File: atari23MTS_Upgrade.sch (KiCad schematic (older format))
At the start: 37 parts, among them P1 CONN_01X01, P2 CONN_01X01, P3 CONN_01X01, P4 CONN_01X01, P5 CONN_01X01, SW1 SW_PUSH, U1 NCP1117ST33T3G, U2 STM32F401RCTx

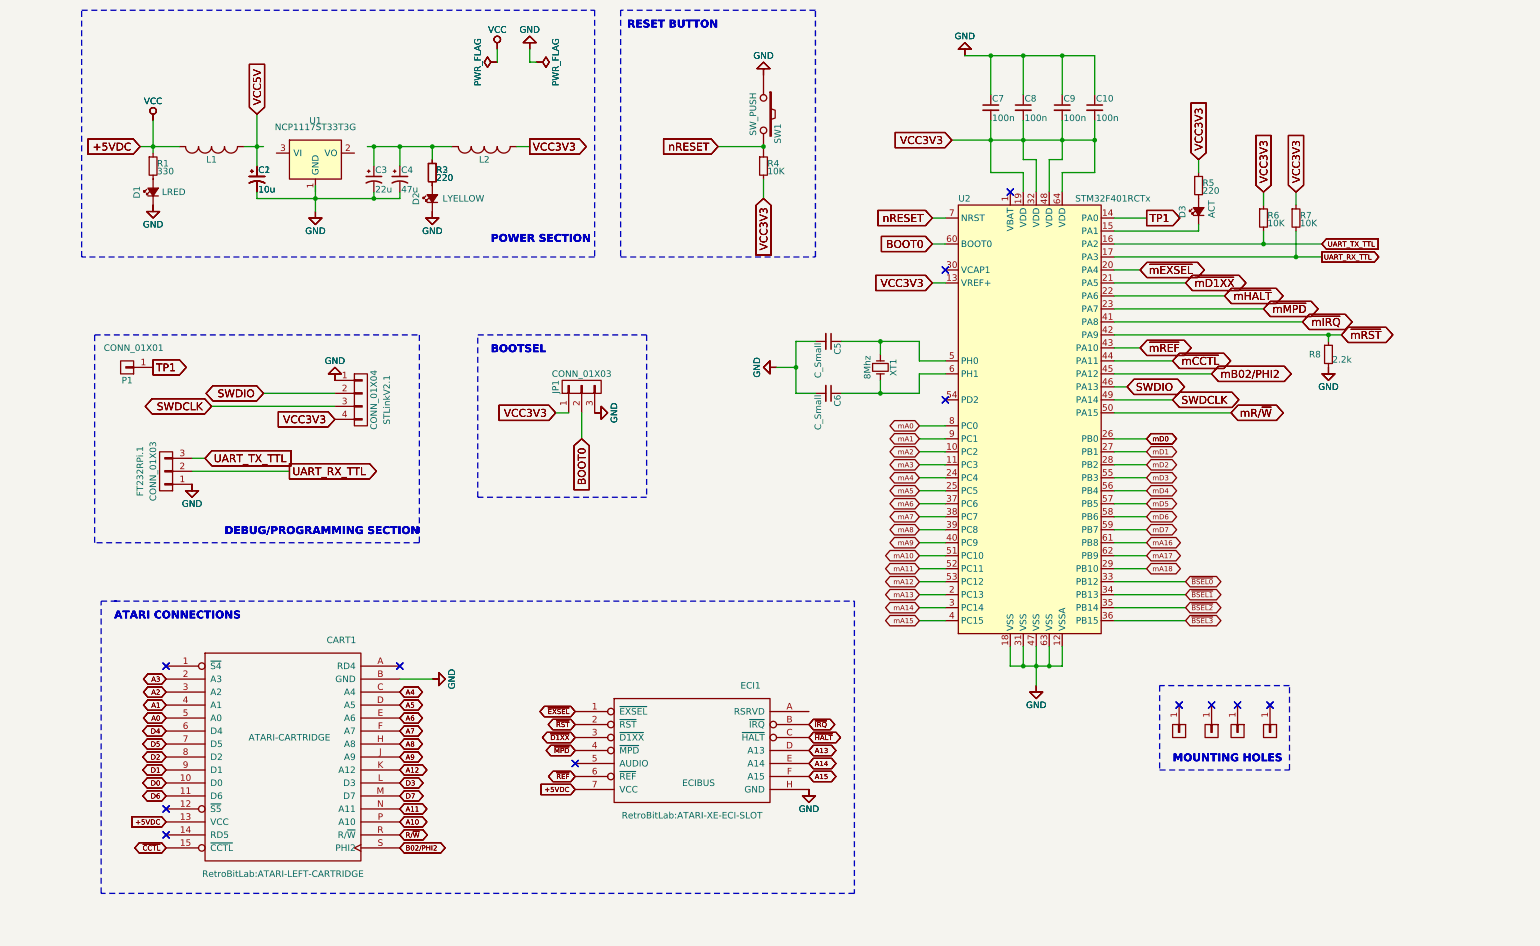
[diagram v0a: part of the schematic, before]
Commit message: modified logic & added pcb
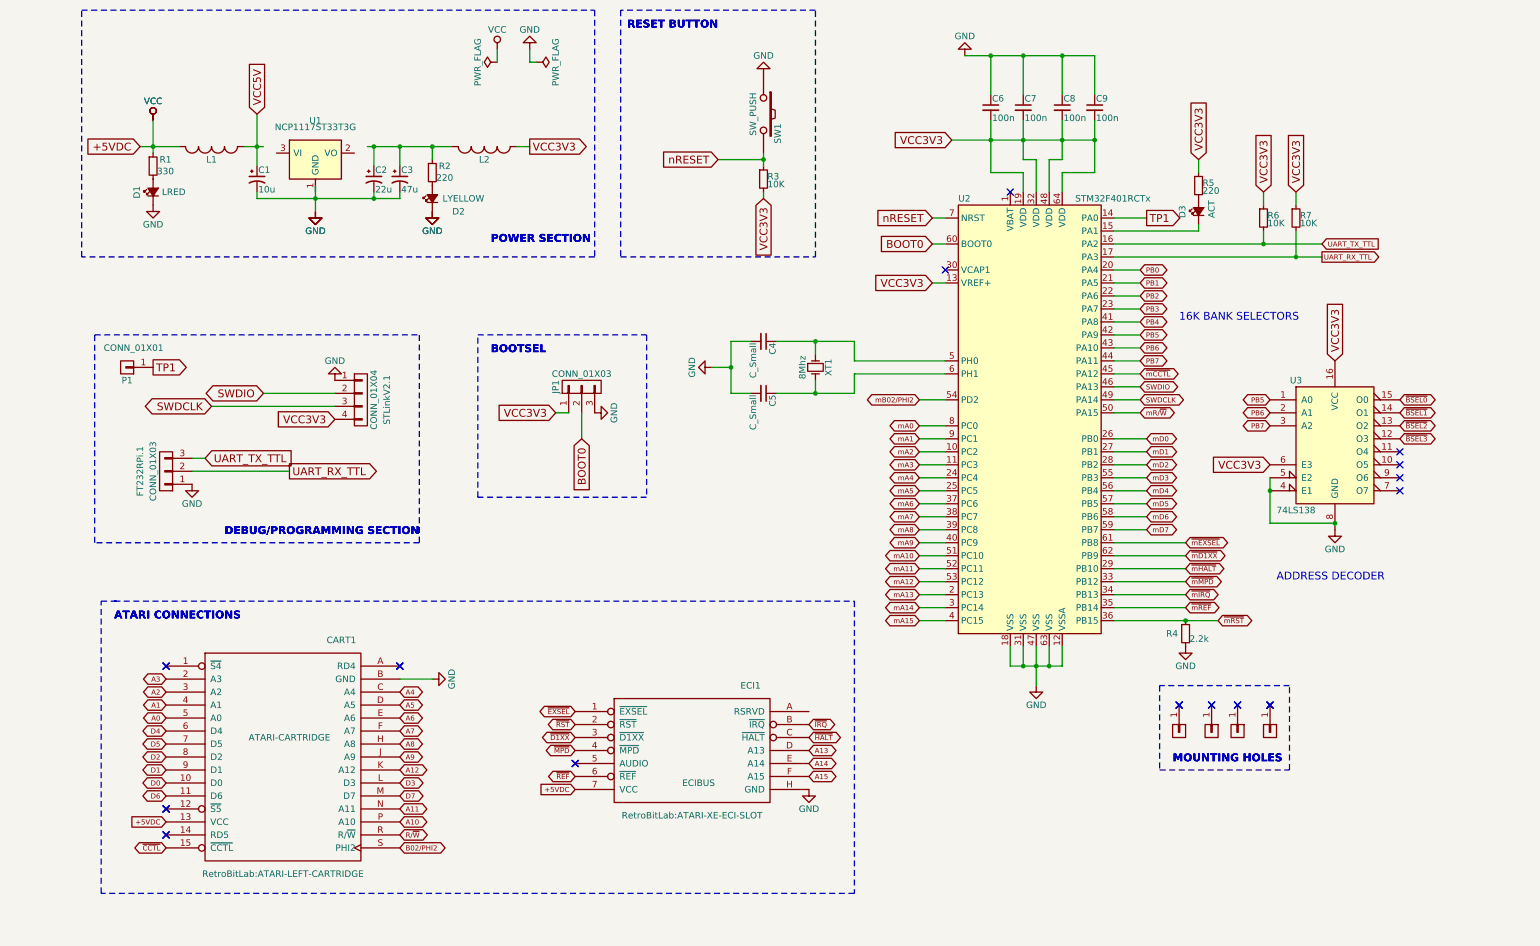
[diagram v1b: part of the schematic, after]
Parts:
- removed C1: 10u, Capacitors_SMD:c_elec_5x5.3, symbol CP1_Small
- removed R2: 220, Resistors_SMD:R_1206_HandSoldering, symbol R_Small
- added U3: 74LS138, Housings_SSOP:TSSOP-16_4.4x5mm_Pitch0.65mm, symbol 74LS138
- renumbered C2 to C1, C3 to C2, C4 to C3, C5 to C4, C6 to C5, C7 to C6, C8 to C7, C9 to C8, C10 to C9, R3 to R2, R4 to R3, R8 to R4
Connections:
- net mA16 is gone; now on net ~mEXSEL: U2.61 (PB8)
- net mA17 is gone; now on net ~mD1XX: U2.62 (PB9)
- net mA18 is gone; now on net ~mHALT: U2.29 (PB10)
- net GND: now also U3.8 (GND)
- net VCC3V3: now also U3.16 (VCC), U3.6 (E3)
- net mB02/PHI2: now also U2.54 (PD2); no longer U2.45 (PA12)
- net nRESET: now also R3.1, SW1.2
- net ~BSEL0: now also U3.15 (O0); no longer U2.33 (PB12)
- net ~BSEL1: now also U3.14 (O1); no longer U2.34 (PB13)
- net ~BSEL2: now also U3.13 (O2); no longer U2.35 (PB14)
- net ~BSEL3: now also U3.12 (O3); no longer U2.36 (PB15)
- net ~mCCTL: now also U2.45 (PA12); no longer U2.44 (PA11)
- net ~mD1XX: no longer U2.21 (PA5)
- net ~mEXSEL: no longer U2.20 (PA4)
- net ~mHALT: no longer U2.22 (PA6)
- net ~mIRQ: now also U2.34 (PB13); no longer U2.41 (PA8)
- net ~mMPD: now also U2.33 (PB12); no longer U2.23 (PA7)
- net ~mREF: now also U2.35 (PB14); no longer U2.43 (PA10)
- net ~mRST: now also U2.36 (PB15); no longer U2.42 (PA9)
- new net: U3.4 (E1), U3.5 (E2)
- new net PB0: U2.20 (PA4)
- new net PB1: U2.21 (PA5)
- new net PB2: U2.22 (PA6)
- new net PB3: U2.23 (PA7)
- new net PB4: U2.41 (PA8)
- new net PB5: U2.42 (PA9), U3.1 (A0)
- new net PB6: U2.43 (PA10), U3.2 (A1)
- new net PB7: U2.44 (PA11), U3.3 (A2)
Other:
- note added: "16K BANK SELECTORS"
- note added: "ADDRESS DECODER"
- moved on the sheet: C4, C5, R3, R4, XT1
